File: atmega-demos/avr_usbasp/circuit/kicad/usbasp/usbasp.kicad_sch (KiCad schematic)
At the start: 22 parts, among them J1 Conn_01x06_Pin, J2 USB_B_Mini, SW1 SW_Push, SW2 SW_Push, U1 ATmega8A-A, Y1 12MHz

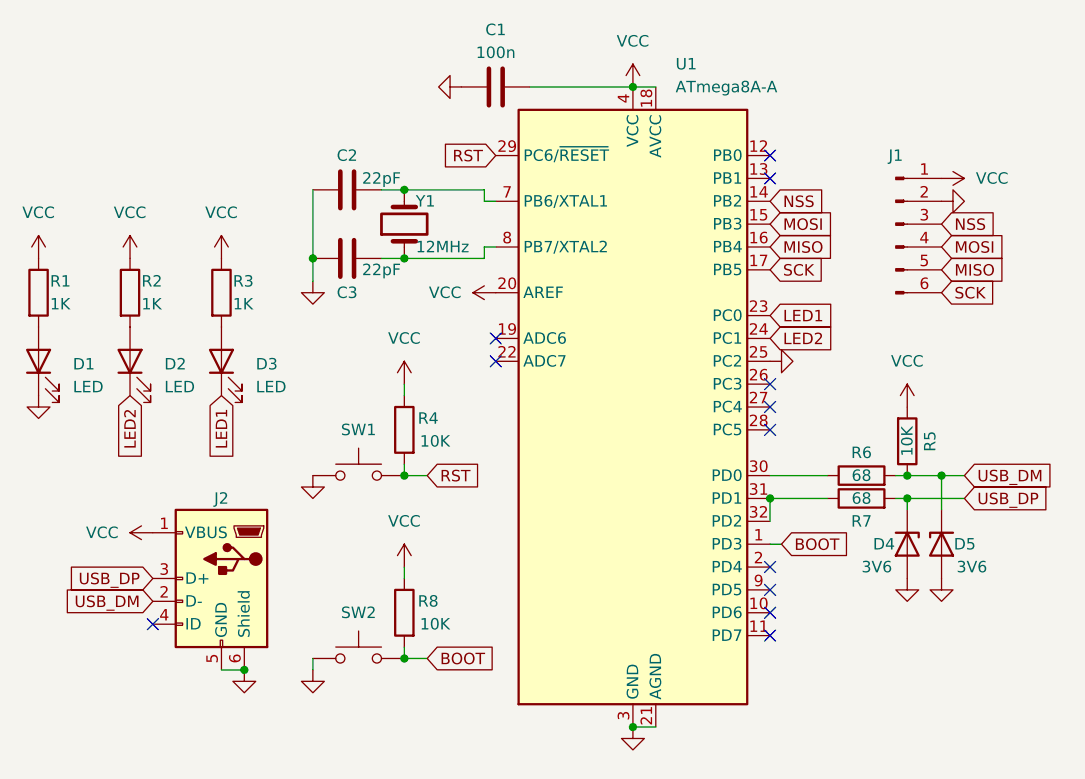
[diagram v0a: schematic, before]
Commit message: USBAsp PCB
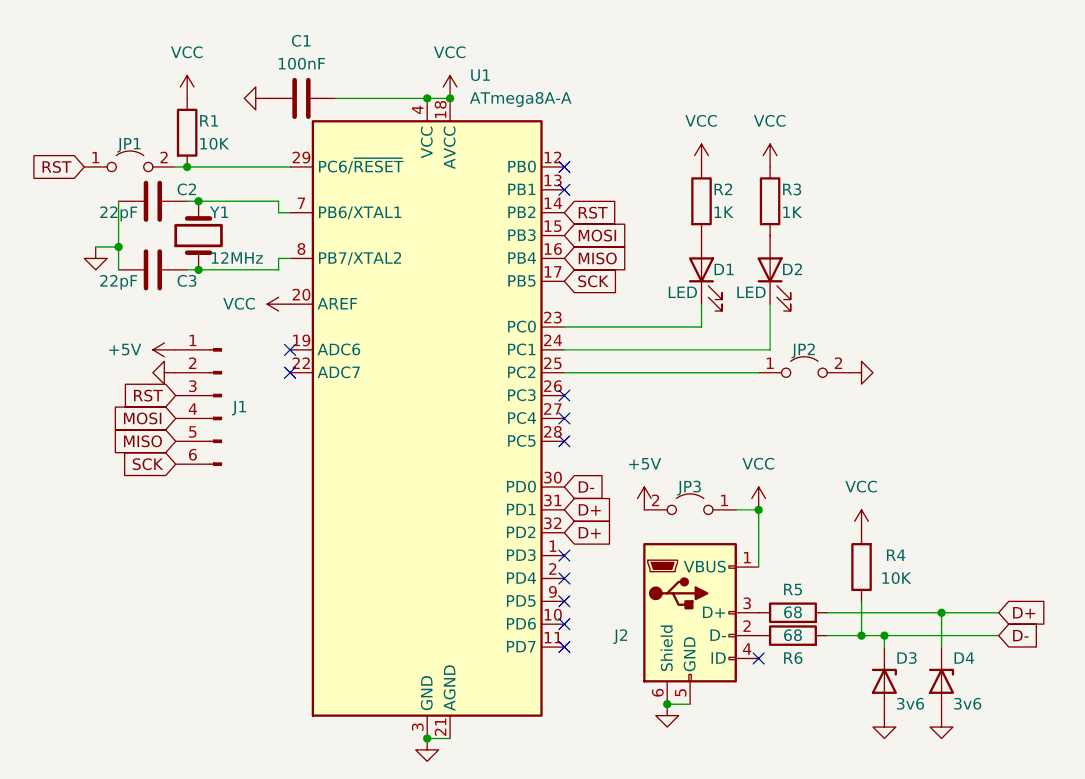
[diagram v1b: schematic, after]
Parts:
- removed D3: LED, LED_SMD:LED_0805_2012Metric_Pad1.15x1.40mm_HandSolder, symbol Device:LED
- removed D5: 3V6, Diode_SMD:D_SOD-323, symbol Device:D_Zener
- removed R7: 68, Resistor_SMD:R_0805_2012Metric_Pad1.20x1.40mm_HandSolder, symbol Device:R
- removed R8: 10K, Resistor_SMD:R_0805_2012Metric_Pad1.20x1.40mm_HandSolder, symbol Device:R
- removed SW1, SW2: SW_Push, Button_Switch_SMD:SW_Tactile_SPST_NO_Straight_CK_PTS636Sx25SMTRLFS, symbol Switch:SW_Push
- added D3: 3v6, Diode_SMD:D_SOD-323, symbol Device:D_Zener
- added JP1, JP2, JP3: Jumper_2_Open, Jumper:SolderJumper-2_P1.3mm_Open_RoundedPad1.0x1.5mm, symbol Jumper:Jumper_2_Open
- C1: value 100n -> 100nF
- D4: value 3V6 -> 3v6
- J1: footprint Connector_PinHeader_2.54mm:PinHeader_1x06_P2.54mm_Vertical -> Connector_PinHeader_2.00mm:PinHeader_1x06_P2.00mm_Vertical
- R1: value 1K -> 10K
- R5: value 10K -> 68
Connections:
- net NSS is gone; now on net RST: J1.3 (Pin_3), U1.14 (PB2)
- net GND: now also D3.2 (A), JP2.2 (B); no longer D1.1 (K), U1.25 (PC2)
- net RST: now also JP1.1 (A); no longer R4.2, U1.29 (PC6/~{RESET})
- net VCC: now also R4.2, JP3.1 (A); no longer J1.1 (Pin_1), R4.1, R5.2
- net D+: now reaches U1.31 (PD1), U1.32 (PD2)
- net D+: now also D4.1 (K), R5.2
- net at D1.2 (A): now also R2.2; no longer R1.2
- net at R6.1: now also J2.2 (D-); no longer U1.30 (PD0)
- net at D2.2 (A): now also R3.2; no longer R2.2
- net BOOT: no longer names the net of U1.1 (PD3)
- net LED1: no longer names the net of U1.23 (PC0)
- net LED1: now also D1.1 (K)
- net LED2: no longer names the net of D2.1 (K), U1.24 (PC1)
- removed net USB_DM: J2.2 (D-), R5.1, R6.2
- net USB_DP: no longer names the net of J2.3 (D+)
- net USB_DP: now also R5.1; no longer D4.1 (K)
- new net: JP2.1 (A), U1.25 (PC2)
- new net: JP1.2 (B), R1.2, U1.29 (PC6/~{RESET})
- new net +5V: J1.1 (Pin_1), JP3.2 (B)
- new net D-: D3.1 (K), R4.1, R6.2, U1.30 (PD0)
- no-connect marks 12 -> 13
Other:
- title: ATMega8 Minimum System -> USBAsp
